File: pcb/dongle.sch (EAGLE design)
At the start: 11 parts, among them IC1 ATSAMD21E18A-AFT, IC2 MCP73831T-2ACI/OT, IC3 IC_XC8107AC20MR-G

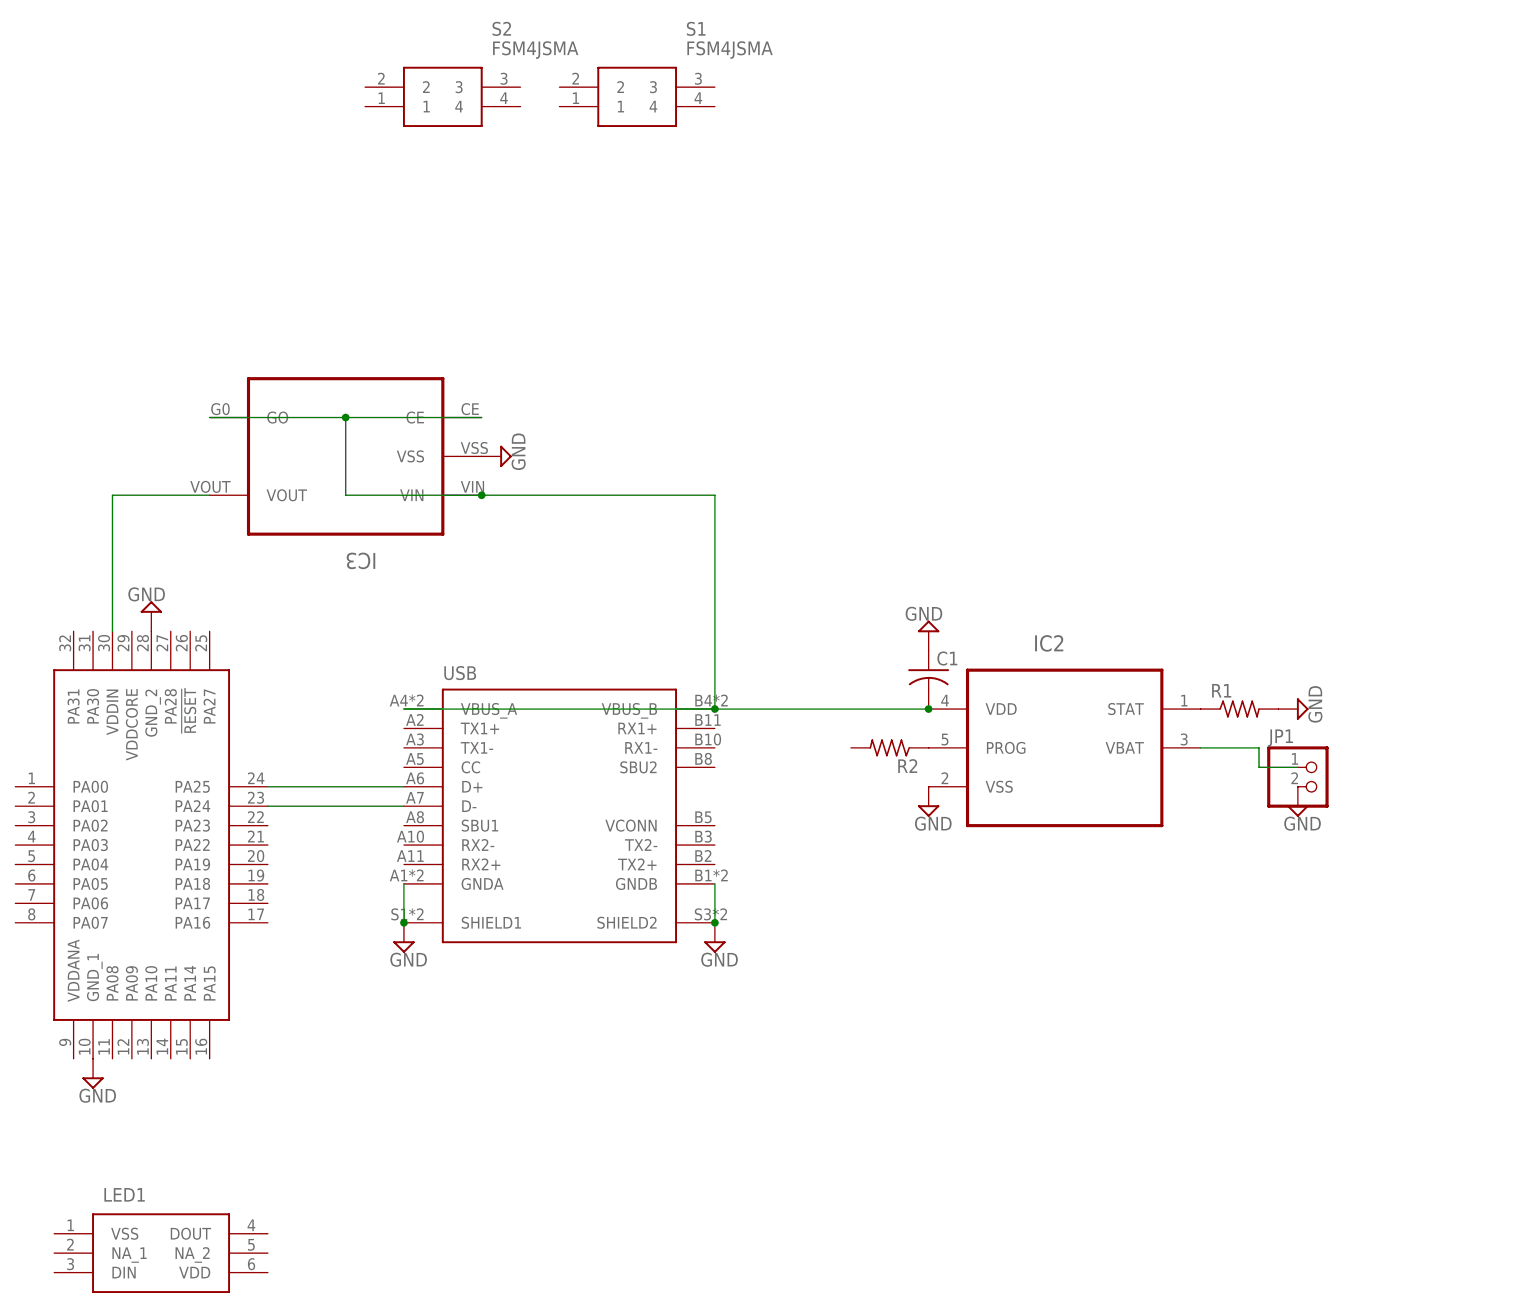
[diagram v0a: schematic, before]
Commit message: Lots of all around work on the code and board
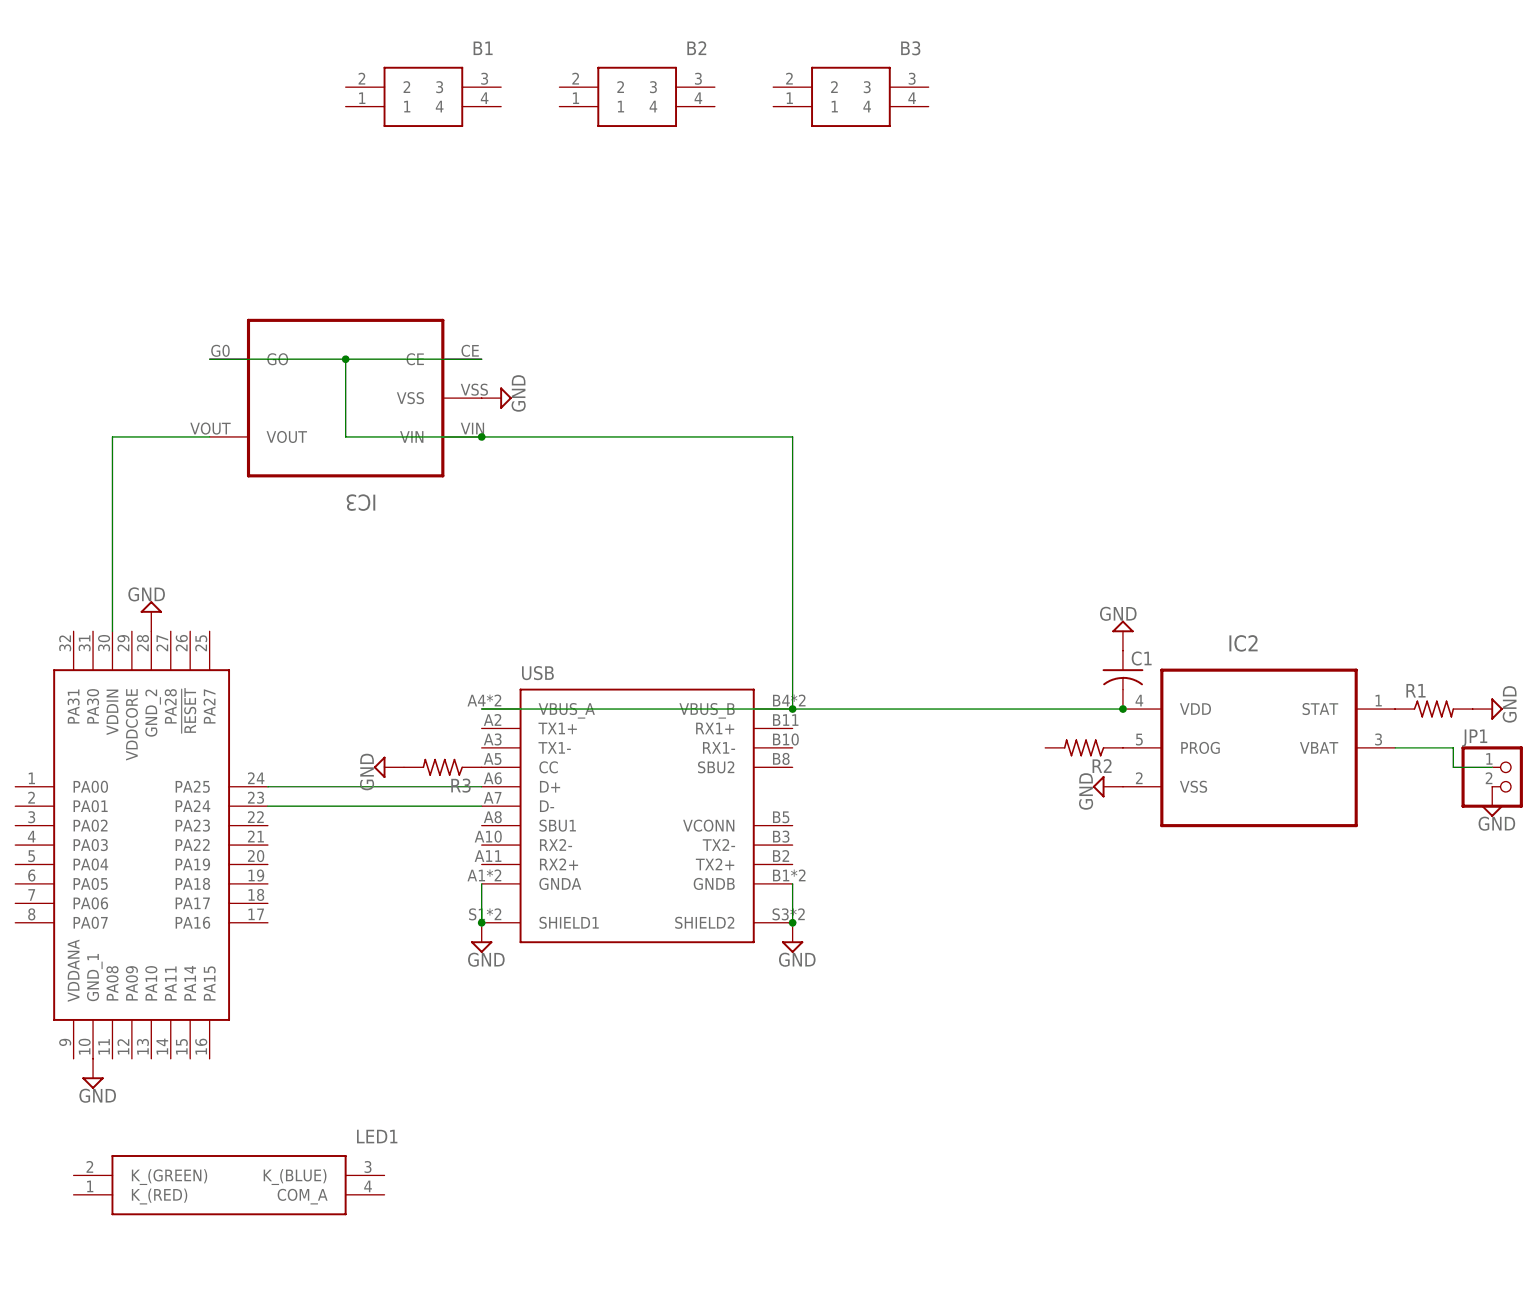
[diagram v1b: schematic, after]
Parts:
- removed S2: FSM4JSMA, FSM4JSMA:FSM4JSMA
- added B1, B3: FSM4JSMA, FSM4JSMA:FSM4JSMA
- added R3: (no value), rcl:R-US_R0805
- LED1: value SMD-LX5050RGB-TR -> ASMB-MTB1-0B3A2; device SMD-LX5050RGB-TR:SMD-LX5050RGB-TR -> SamacSys_Parts:ASMB-MTB1-0B3A2
- renumbered S1 to B2
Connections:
- new net CC: R3.1, USB.CC
- net GND: now also R3.2
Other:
- moved on the sheet: C1, IC2, IC3, JP1, R1, R2, USB
